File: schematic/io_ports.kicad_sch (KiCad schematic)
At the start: 2 parts, among them J4 Cartridge Port

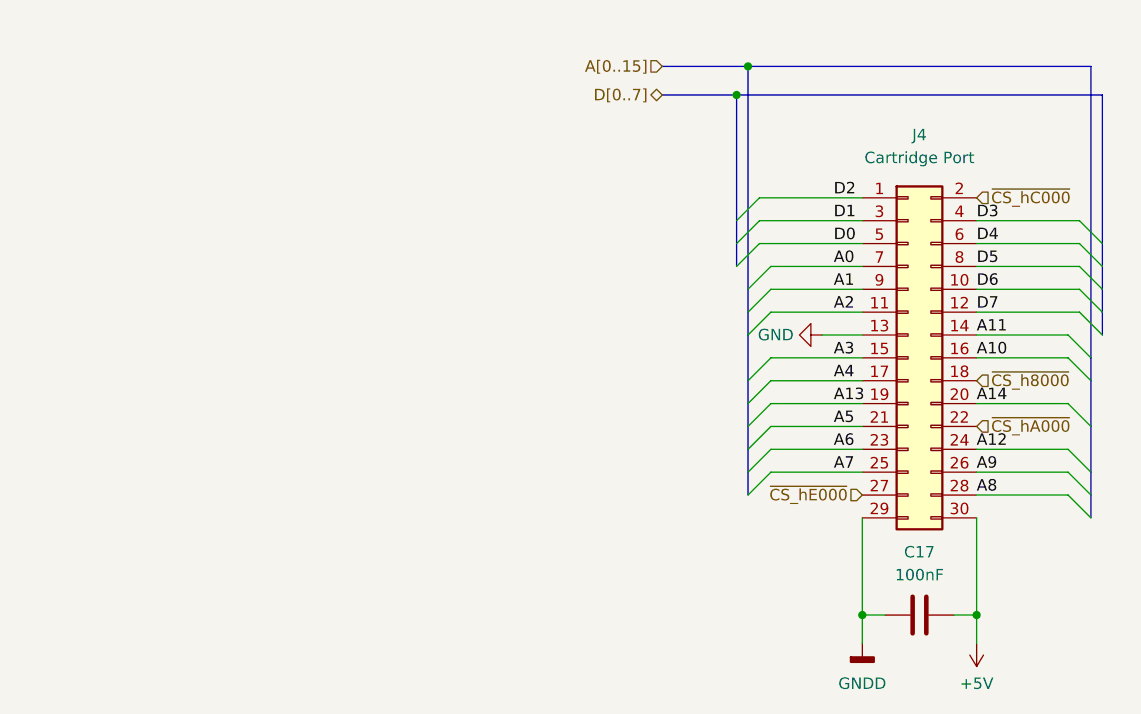
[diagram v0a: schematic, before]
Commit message: update for release, correct documents, and update readme
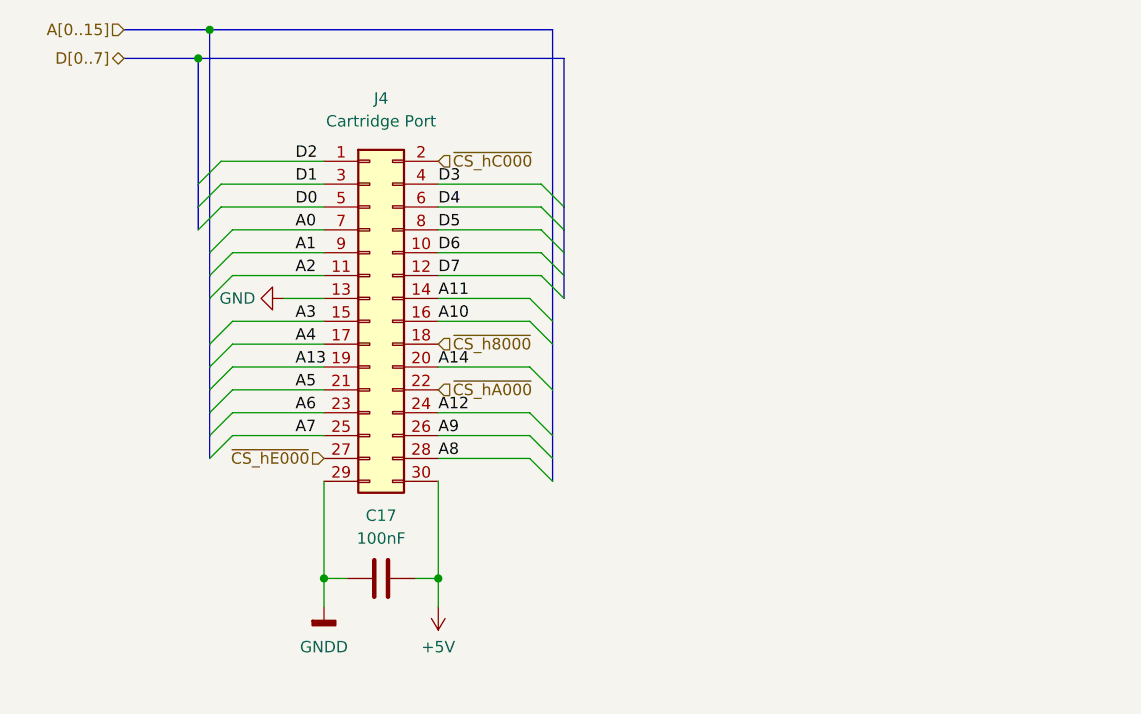
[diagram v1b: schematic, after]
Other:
- moved on the sheet: C17, J4
